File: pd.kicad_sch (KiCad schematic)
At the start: 1 part

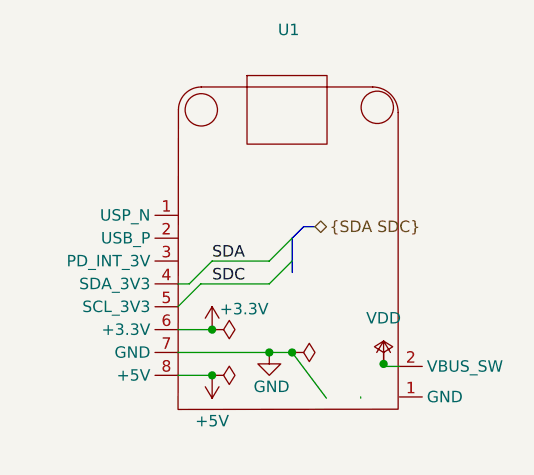
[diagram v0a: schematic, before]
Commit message: begin pcb
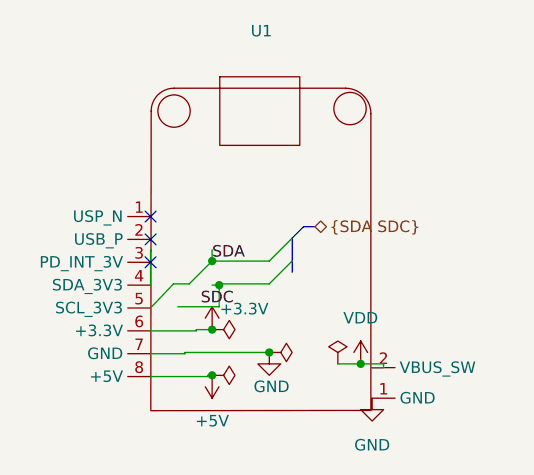
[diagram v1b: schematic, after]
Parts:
- U1: footprint (none) -> Audio_Module:rotopd
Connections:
- net GND: now also U1.1 (GND)
- net SDA: now also U1.5 (SCL_3V3); no longer U1.4 (SDA_3V3)
- net SDC: no longer U1.5 (SCL_3V3)
- no-connect marks 0 -> 3
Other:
- moved on the sheet: U1
